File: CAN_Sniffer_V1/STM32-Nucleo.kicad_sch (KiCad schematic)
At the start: 2 parts, among them J4 STL Link, U4 NUCLEO-F072RB

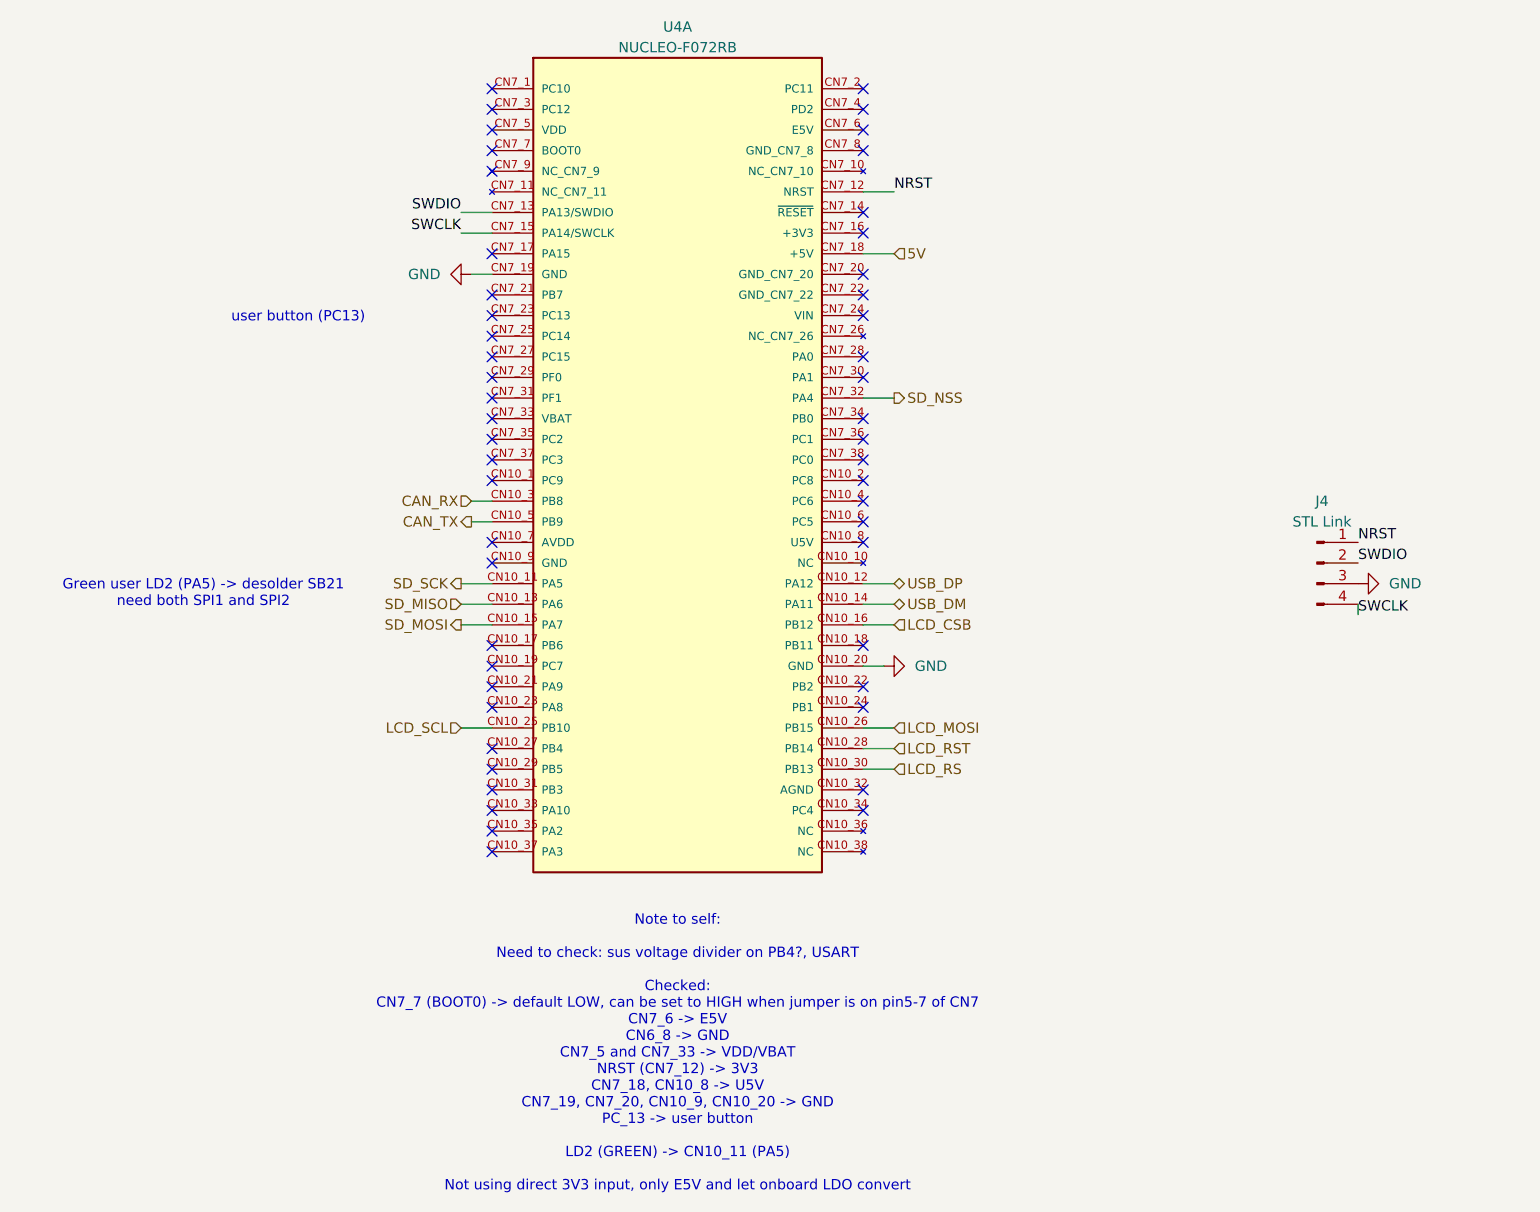
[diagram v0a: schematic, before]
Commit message: iteration 2 routing
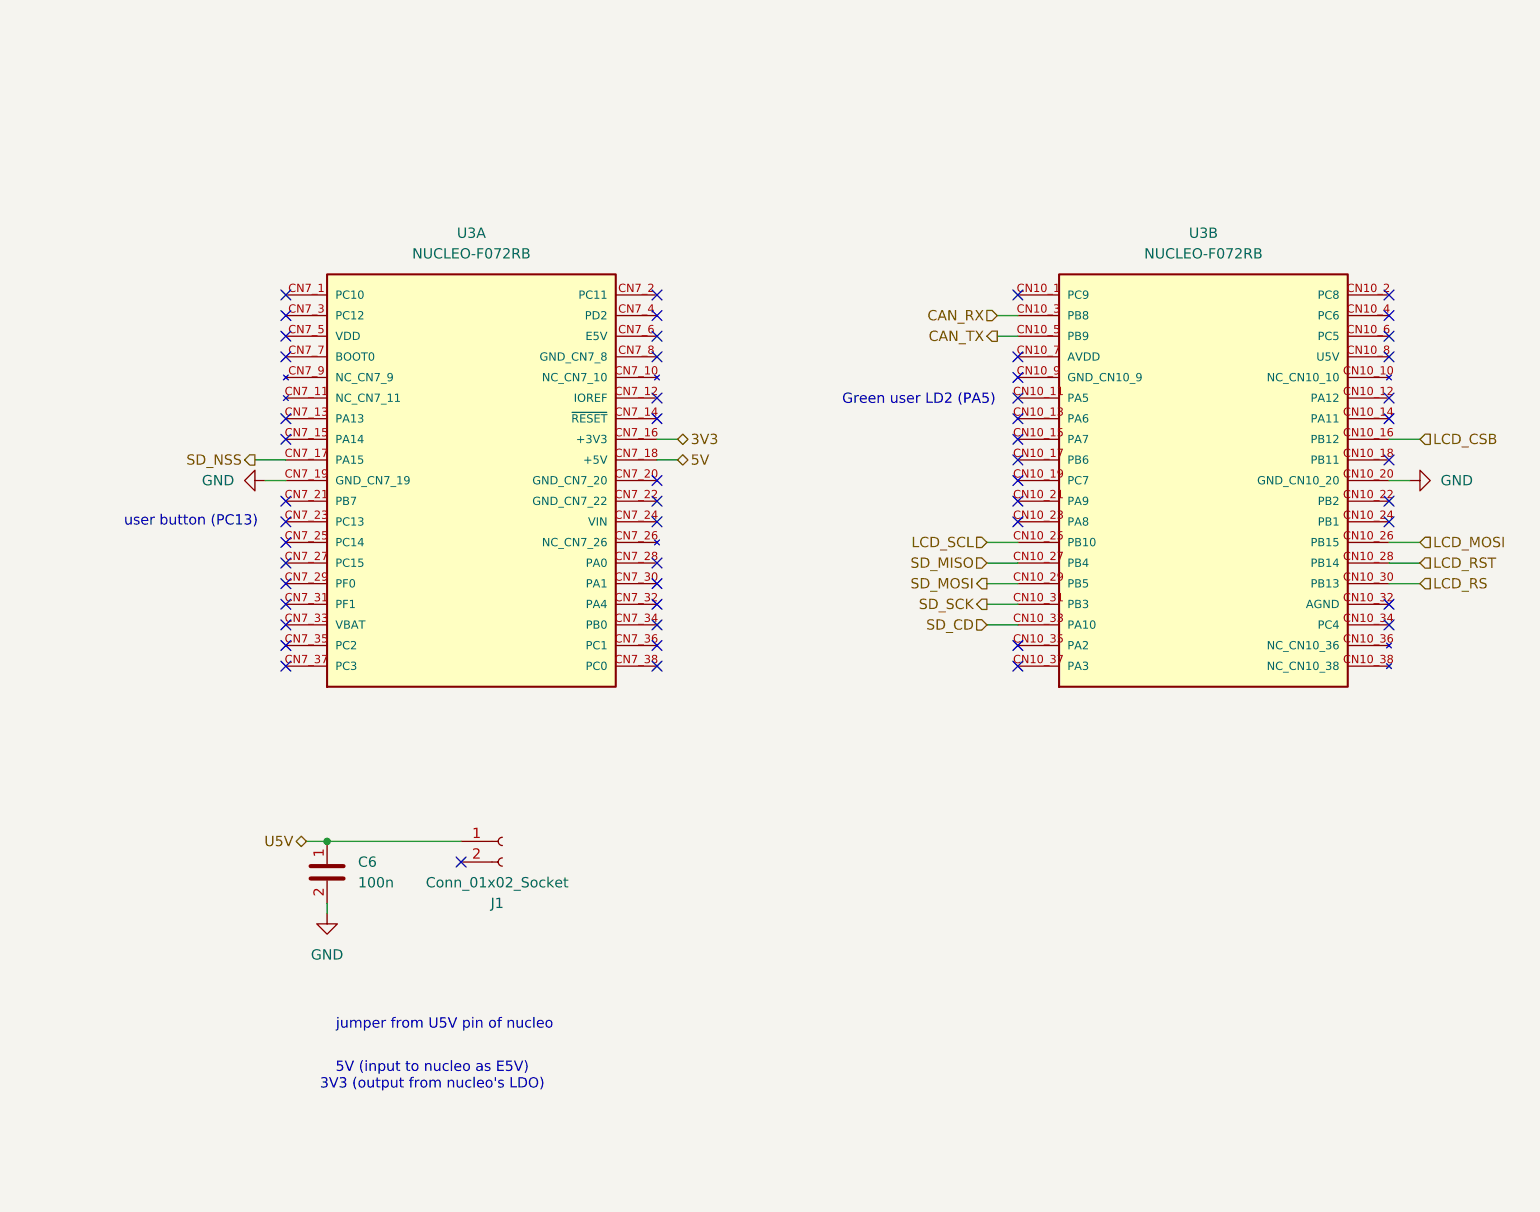
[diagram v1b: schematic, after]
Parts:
- removed J4: STL Link, Connector_PinHeader_2.54mm:PinHeader_1x04_P2.54mm_Vertical, symbol Connector:Conn_01x04_Pin
- removed U4: NUCLEO-F072RB, STM32F0_breakout:MODULE_NUCLEO-F072RB, symbol NUCLEO-F072RB:NUCLEO-F072RB
- added C6: 100n, Capacitor_SMD:C_0805_2012Metric_Pad1.18x1.45mm_HandSolder, symbol bfr_capacitors:08051C104KAT4A
- added J1: Conn_01x02_Socket, Connector_PinHeader_2.54mm:PinHeader_1x02_P2.54mm_Vertical, symbol Connector:Conn_01x02_Socket
- added U3: NUCLEO-F072RB, STM32F0_breakout:MODULE_NUCLEO-F072RB, symbol NUCLEO-F072RB:NUCLEO-F072RB
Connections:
- net 5V: now also U3.CN7_18 (+5V)
- net CAN_RX: now also U3.CN10_3 (PB8)
- net CAN_TX: now also U3.CN10_5 (PB9)
- net GND: now also C6.2, U3.CN10_20 (GND_CN10_20), U3.CN7_19 (GND_CN7_19)
- net LCD_CSB: now also U3.CN10_16 (PB12)
- net LCD_MOSI: now also U3.CN10_26 (PB15)
- net LCD_RS: now also U3.CN10_30 (PB13)
- net LCD_RST: now also U3.CN10_28 (PB14)
- net LCD_SCL: now also U3.CN10_25 (PB10)
- net SD_MISO: now also U3.CN10_27 (PB4)
- net SD_MOSI: now also U3.CN10_29 (PB5)
- net SD_NSS: now also U3.CN7_17 (PA15)
- net SD_SCK: now also U3.CN10_31 (PB3)
- new net 3V3: U3.CN7_16 (+3V3)
- new net SD_CD: U3.CN10_33 (PA10)
- new net U5V: C6.1, J1.1 (Pin_1)
- no-connect marks 51 -> 54
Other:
- note added: "5V (input to nucleo as E5V) 3V3 (output from nucleo's LDO)"
- note added: "Green user LD2 (PA5)"
- note added: "jumper from U5V pin of nucleo"
- note removed: "Green user LD2 (PA5) -> desolder SB21 need both SPI1 and SPI2"
- note removed: "Note to self: Need to check: sus voltage divider on PB4?, USART Checked: CN7_7 (BOOT0) -> default LOW, can be set to HIGH when jumper is on pin5-7 of CN7 CN7_6 -> E5V CN6_8 -> GND CN7_5 and CN7_33 -> VDD/VBAT NRST (CN7_12) -> 3V3 CN7_18, CN10_8 -> U5V CN7_19, CN7_20, CN10_9, CN10_20 -> GND PC_13 -> user button LD2 (GREEN) -> CN10_11 (PA5) Not using direct 3V3 input, only E5V and let onboard LDO c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"
